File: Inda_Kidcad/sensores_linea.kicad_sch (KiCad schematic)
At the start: 20 parts, among them J4 Conn_01x03_Pin, J5 Conn_01x03_Pin, J6 Conn_01x03_Pin, J7 Conn_01x03_Pin, U10 QRE111GR, U11 QRE111GR, U8 QRE111GR, U9 QRE111GR

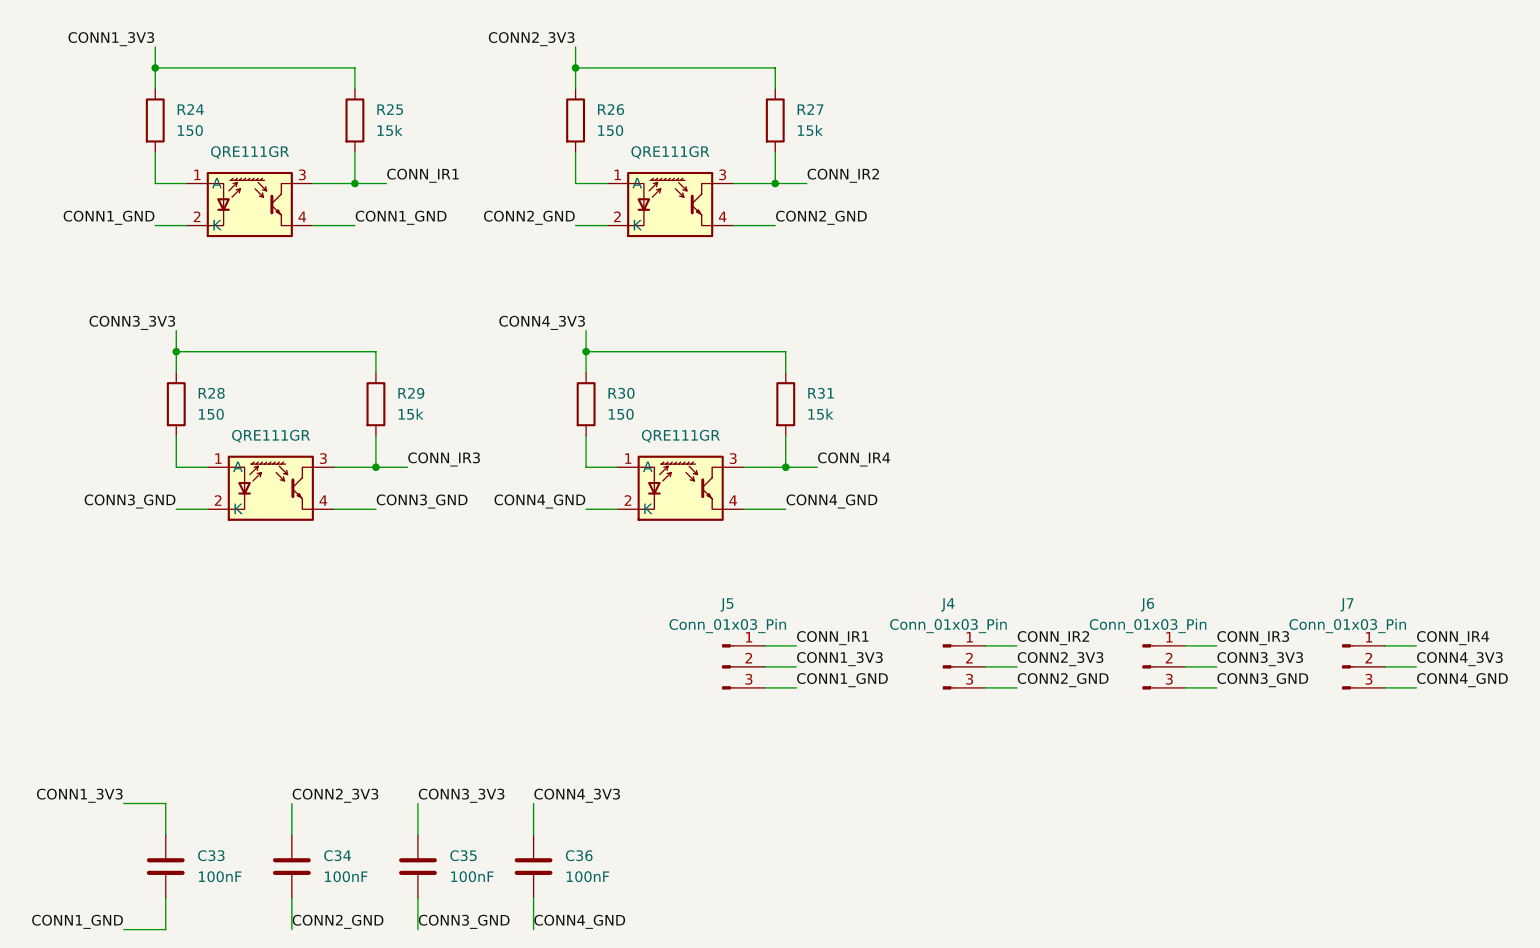
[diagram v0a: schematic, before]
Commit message: Version 2 De Sumo Inda
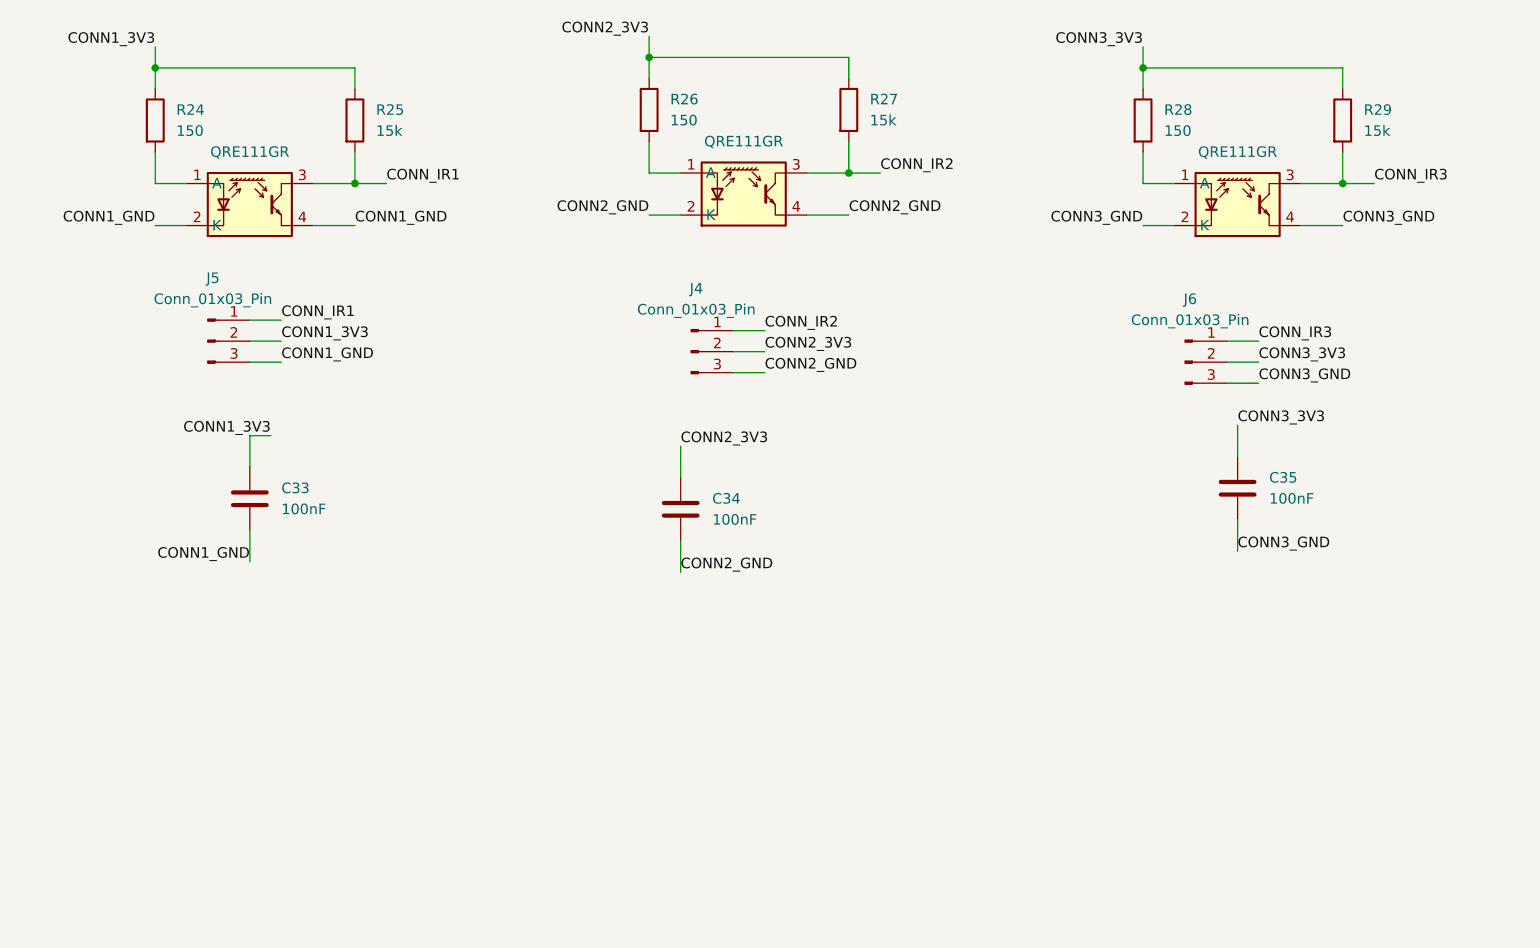
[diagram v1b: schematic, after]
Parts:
- removed C36: 100nF, Capacitor_SMD:C_0603_1608Metric_Pad1.08x0.95mm_HandSolder, symbol Device:C
- removed J7: Conn_01x03_Pin, Footprint:CONN_SMD_01X03_IR, symbol Connector:Conn_01x03_Pin
- removed R30: 150, Resistor_SMD:R_0805_2012Metric_Pad1.20x1.40mm_HandSolder, symbol Device:R
- removed R31: 15k, Resistor_SMD:R_0805_2012Metric_Pad1.20x1.40mm_HandSolder, symbol Device:R
- removed U11: QRE111GR, Footprint:QRE1113GR_IR, symbol Micromouse_Library:QRE1113GR
- U10, U8, U9: symbol Micromouse_Library:QRE1113GR -> LIB_Componentes:QRE1113GR
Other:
- moved on the sheet: C33, C34, C35, J4, J5, J6, R26, R27, R28, R29
